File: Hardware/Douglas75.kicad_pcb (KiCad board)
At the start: 2 copper layers, 91.8 x 100.5 mm, 24 parts, among them Q1 IRLZ44N, Q2 IRLZ44N, U2 ESP32-DevKitC, U3 L7805

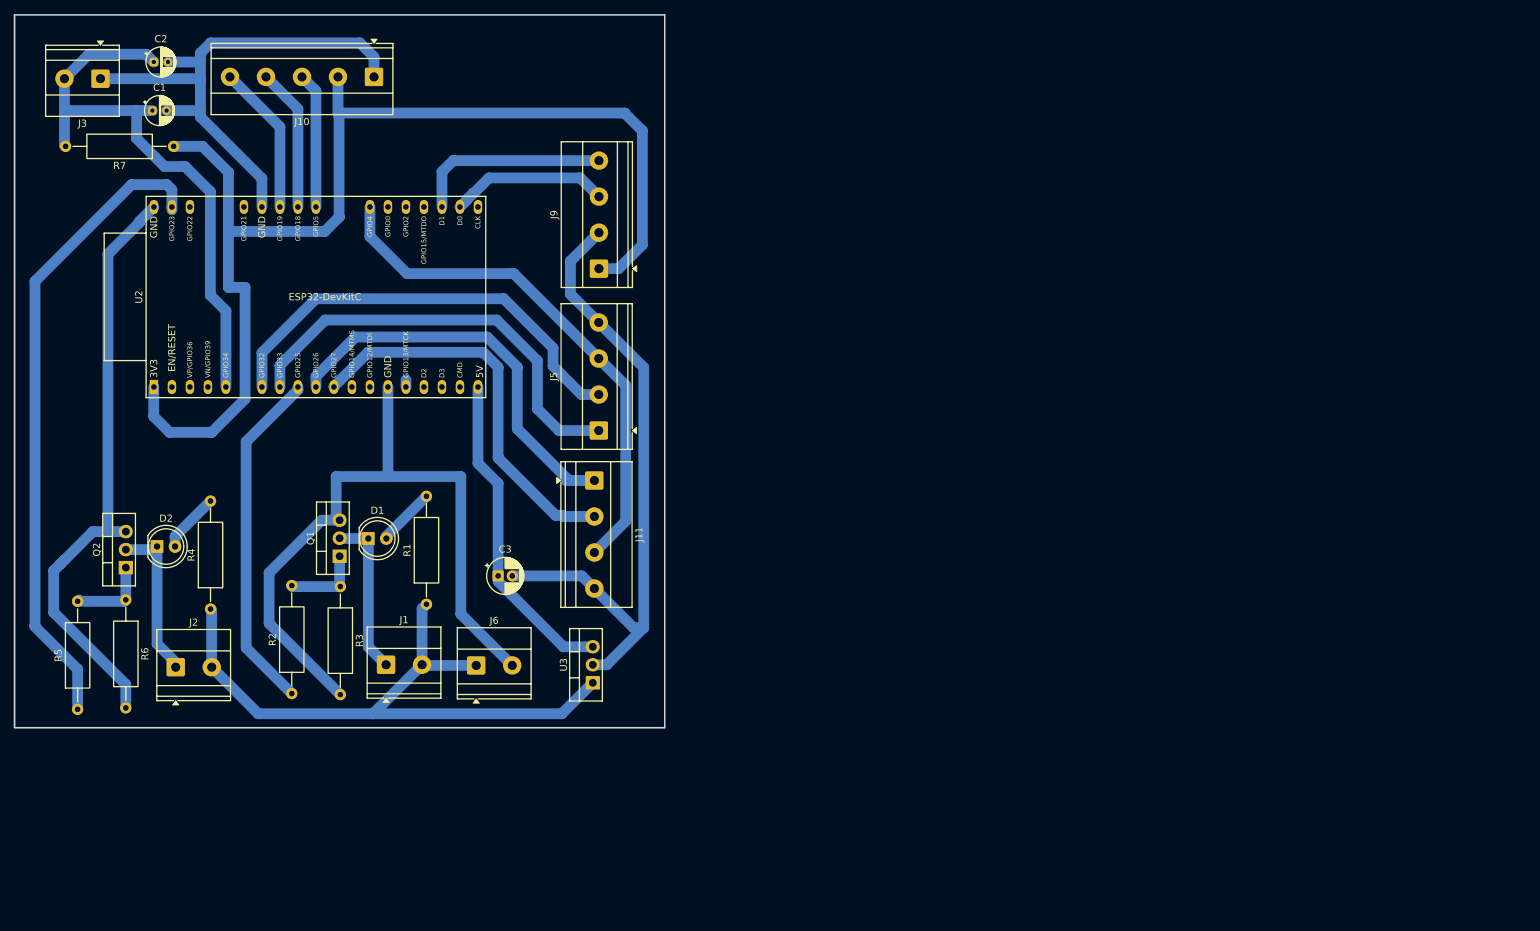
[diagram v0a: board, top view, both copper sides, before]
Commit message: Add files via upload
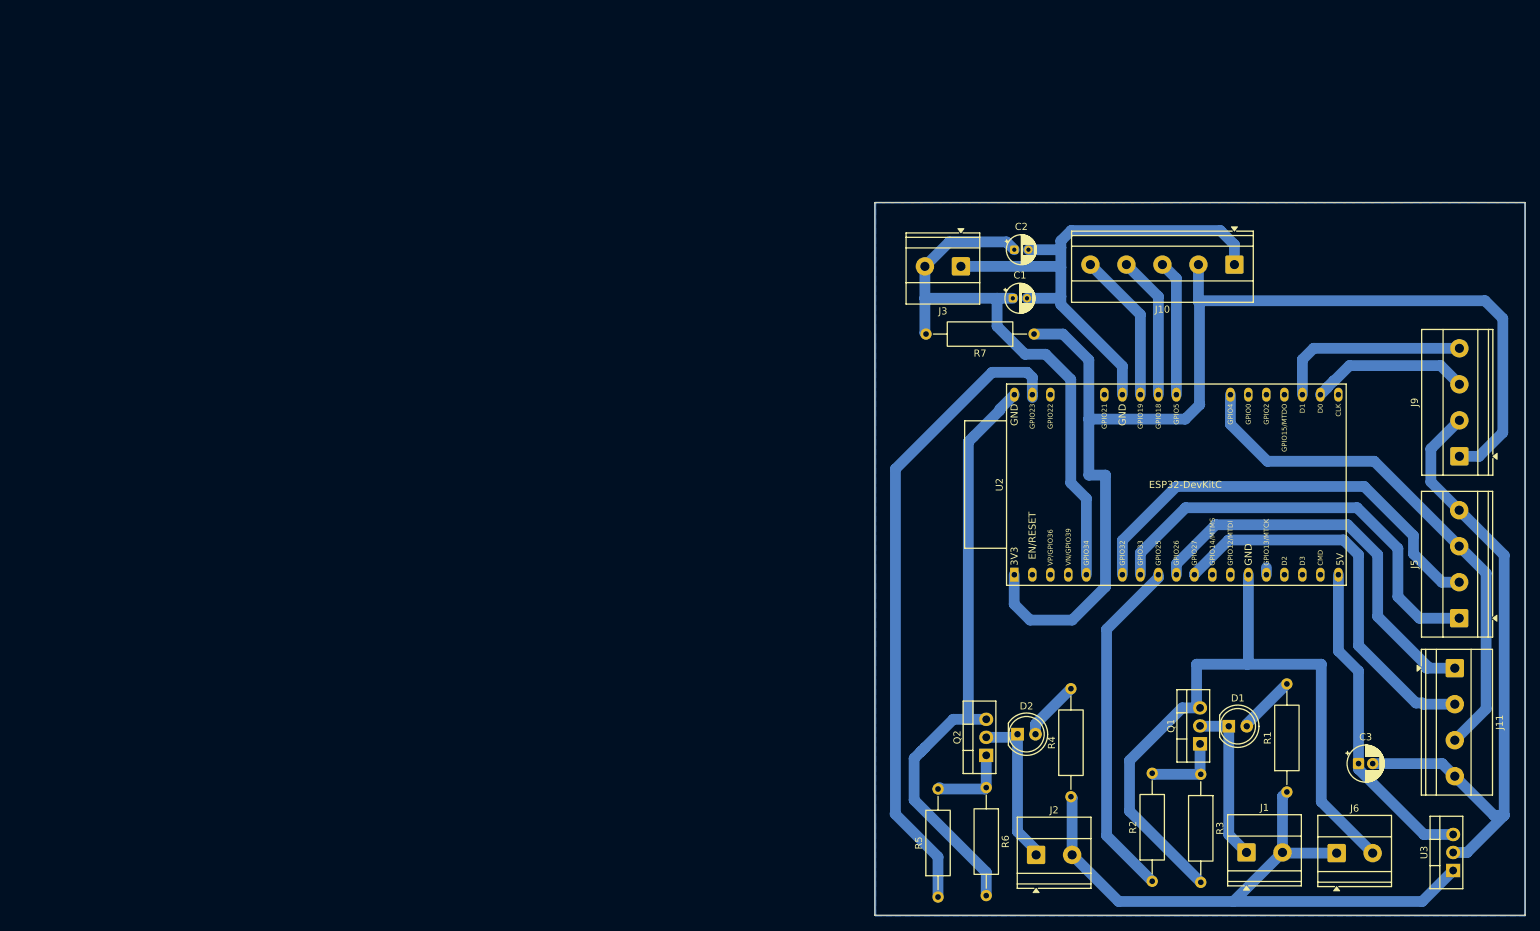
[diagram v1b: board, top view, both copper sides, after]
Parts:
- moved C1 124.2 mm to (198.2, 71.3)
- moved J9 124.2 mm to (261.2, 93.6)
- moved Q1 124.2 mm to (224.6, 134.2)
- moved R1 124.2 mm to (236.8, 140.9)
- moved R2 124.2 mm to (217.8, 153.5)
- moved R4 124.2 mm to (206.4, 141.6)
- moved R5 124.2 mm to (187.6, 155.8)
- moved U3 124.2 mm to (260.3, 152.0)
- moved C2 124.2 mm to (198.4, 64.4)
- moved C3 124.2 mm to (246.9, 136.9)
- moved D1 124.2 mm to (228.6, 131.7)
- moved J1 124.2 mm to (231.1, 149.5)
- moved J10 124.2 mm to (229.4, 66.5)
- moved J3 124.2 mm to (190.8, 66.8)
- moved J6 124.2 mm to (243.8, 149.6)
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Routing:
- added copper zone on B.Cu, net GNDREF
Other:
- board size 91.8 x 100.5 mm -> 91.8 x 100.6 mm
